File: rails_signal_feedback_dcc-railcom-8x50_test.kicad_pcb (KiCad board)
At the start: 2 copper layers, 9 parts, among them J201 Conn_02x05_Odd_Even, Q101 S8550, Q103 S8050, Q104 S8550

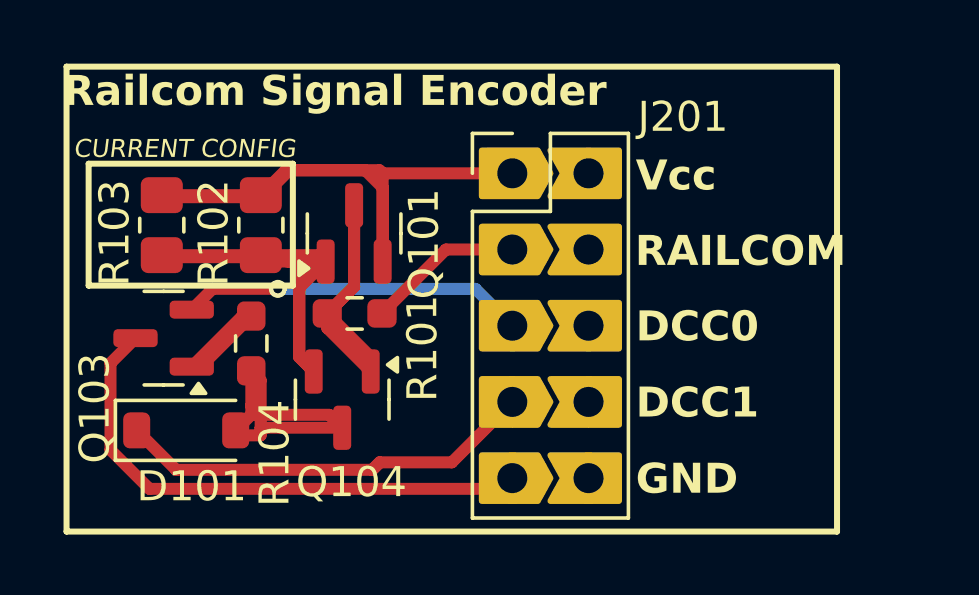
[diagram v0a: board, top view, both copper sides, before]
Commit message: Fix - Test für RC 8x50
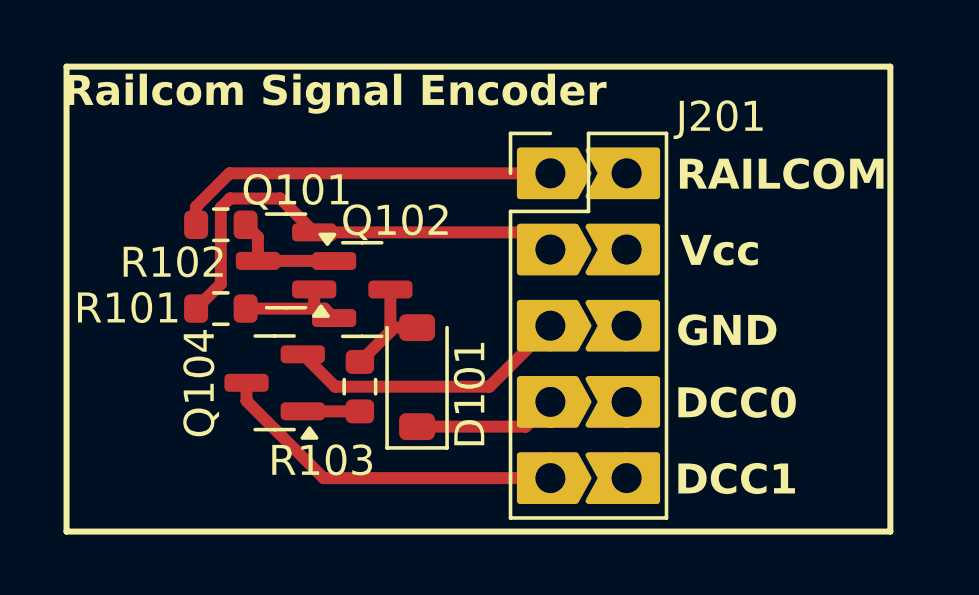
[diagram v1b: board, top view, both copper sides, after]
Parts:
- removed Q103: S8050, xDuinoRail:8x50_SOT-23
- removed R104: 10k, Resistor_SMD:R_0603_1608Metric_Pad0.98x0.95mm_HandSolder
- added Q102: S8550, xDuinoRail:8x50_SOT-23, F.Cu at (131.4, 73.7)
- Q104: value S8550 -> S8050
- R101: value 10k -> 20R; footprint Resistor_SMD:R_0603_1608Metric_Pad0.98x0.95mm_HandSolder -> Resistor_SMD:R_0603_1608Metric
- R102: value 20R -> 10k; footprint Resistor_SMD:R_0805_2012Metric_Pad1.20x1.40mm_HandSolder -> Resistor_SMD:R_0603_1608Metric
- R103: value 1M -> 10k; footprint Resistor_SMD:R_0805_2012Metric_Pad1.20x1.40mm_HandSolder -> Resistor_SMD:R_0603_1608Metric
- moved R103 8.52 mm to (131.3, 77.0), turned to -90 degrees
- moved D101 7.90 mm to (133.2, 76.6), turned to 90 degrees
- moved R101 4.46 mm to (126.7, 74.4), turned to 180 degrees
- moved Q101 2.45 mm to (128.9, 72.8), turned to 180 degrees
- moved Q104 2.32 mm to (128.5, 76.8), turned to 180 degrees
- moved R102 1.33 mm to (126.7, 71.6), turned to 180 degrees
- moved J201 1.27 mm to (137.7, 69.8)
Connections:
- J201 pad 1: /+J_3v3 -> /J_RAILCOM_DATA
- J201 pad 2: /+3V3 -> /RAILCOM_DATA
- J201 pad 3: /J_RAILCOM_DATA -> /+J_3v3
- J201 pad 4: /RAILCOM_DATA -> /+3V3
- Q104 pad 1: /rails_signal_feedback_dcc-railcom-8x50/RC_CURR -> 0
- Q104 pad 2: /rails_signal_feedback_dcc-railcom-8x50/RC_DATA_IN -> Net-(Q104-B)
- Q104 pad 3: /rails_signal_feedback_dcc-railcom-8x50/RC_SIGNAL -> /J_DCC1
- R101 pad 1: /rails_signal_feedback_dcc-railcom-8x50/RC_DATA_IN -> /rails_signal_feedback_dcc-railcom-8x50/RC_CURR
- R101 pad 2: /J_RAILCOM_DATA -> /+J_3v3
- R102 pad 1: /rails_signal_feedback_dcc-railcom-8x50/RC_CURR -> /rails_signal_feedback_dcc-railcom-8x50/RC_DATA_IN
- R102 pad 2: /+J_3v3 -> /J_RAILCOM_DATA
- R103 pad 1: /rails_signal_feedback_dcc-railcom-8x50/RC_CURR -> /rails_signal_feedback_dcc-railcom-8x50/RC_SIGNAL
- R103 pad 2: /+J_3v3 -> Net-(Q104-B)
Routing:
- net /rails_signal_feedback_dcc-railcom-8x50/RC_CURR: track 19.1 -> 3.72 mm
- net /+J_3v3: track 25.4 -> 15.5 mm
- net /J_DCC0: track 14.4 -> 4.79 mm
- net /rails_signal_feedback_dcc-railcom-8x50/RC_DATA_IN: track 13.0 -> 3.92 mm
- net /J_RAILCOM_DATA: track 5.23 -> 12.9 mm
- net /rails_signal_feedback_dcc-railcom-8x50/RC_SIGNAL: track 11.2 -> 3.72 mm
- net /J_DCC1: track 18.2 -> 11.8 mm
- net Net-(Q103-B): track 5.36 -> 0.00 mm
- net 0: track 11.5 -> 9.54 mm, vias 1 -> 0
- net Net-(Q104-B): track 0.00 -> 1.91 mm
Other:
- board text removed: "CURRENT CONFIG"
